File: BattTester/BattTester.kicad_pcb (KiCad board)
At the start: 2 copper layers, 25 parts, among them J1 Battery, J2 SD_Card, J3 PWR, J4 UPDI, Q1 IRLZ44N, U1 LT1286CN8, U2 ATtiny1624-SS, U3 LD1086DT33, U4 LM358AN

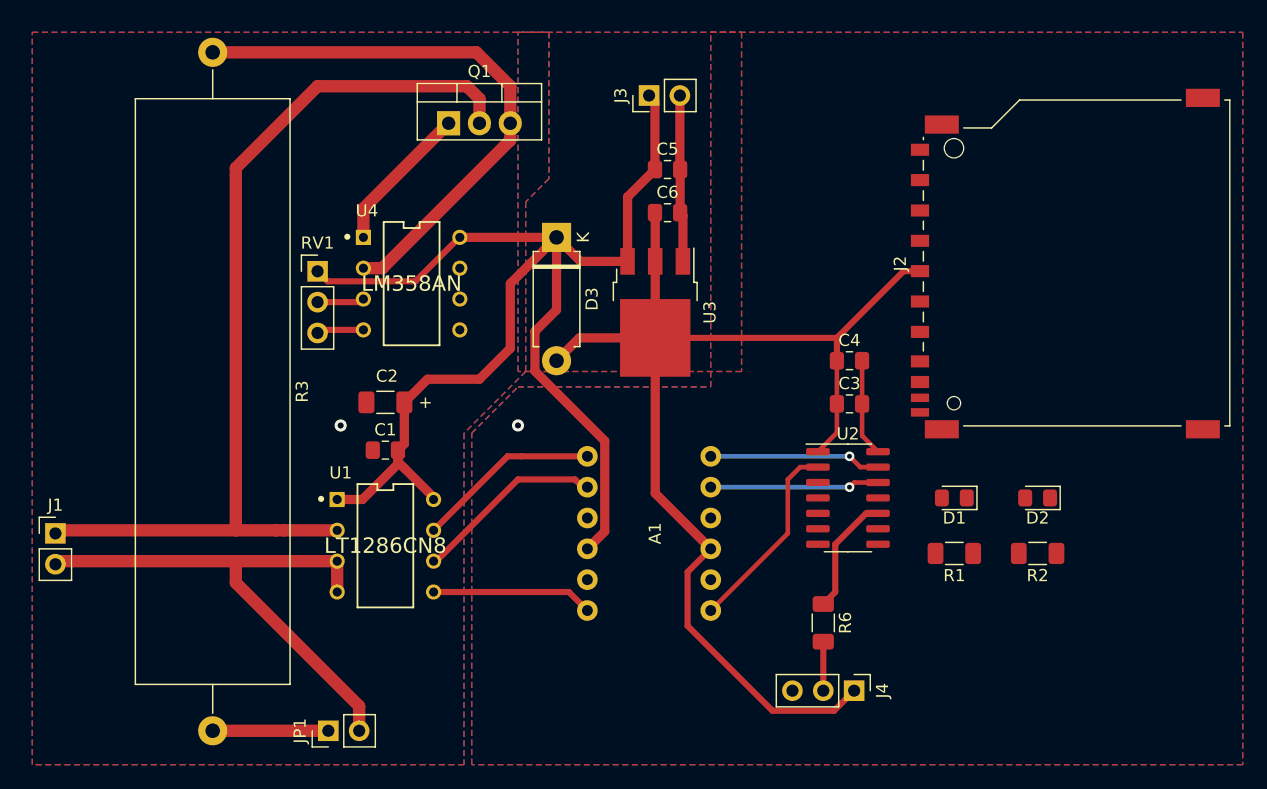
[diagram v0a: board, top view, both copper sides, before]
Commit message: Finish routing
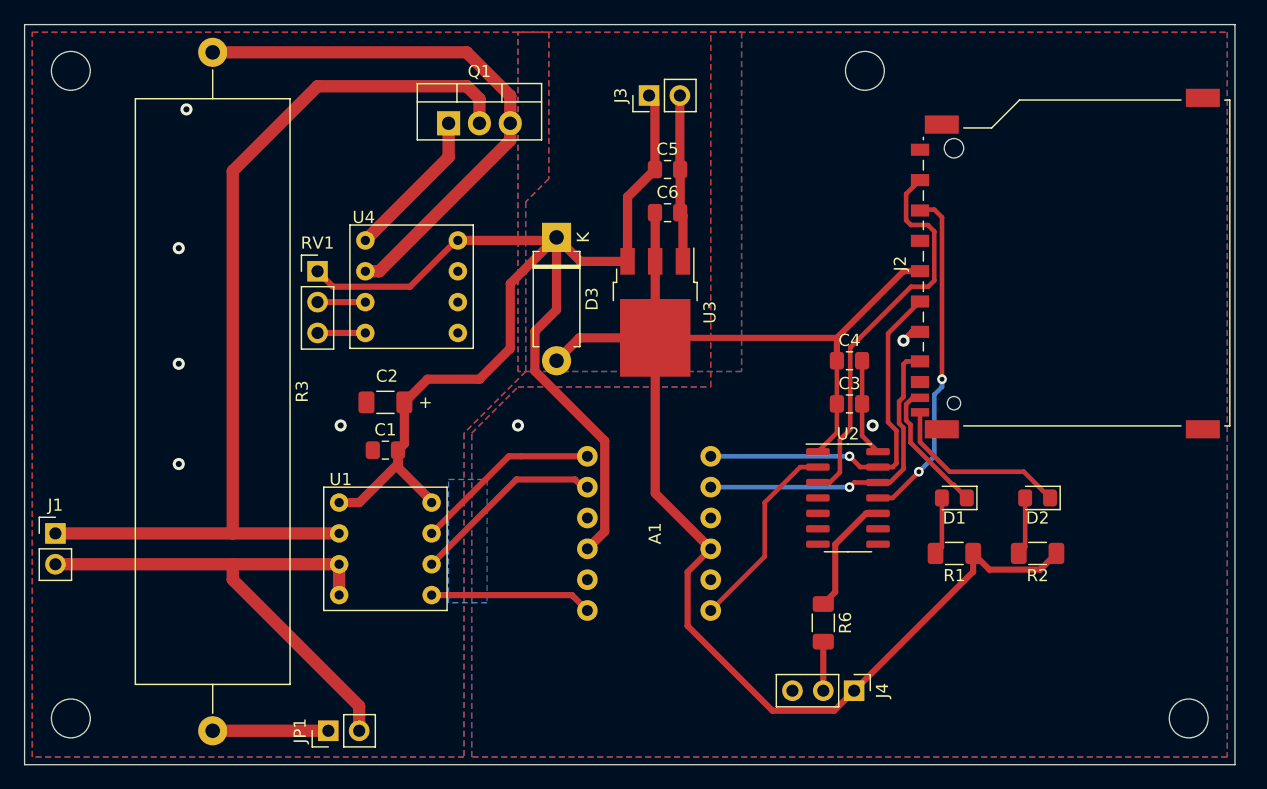
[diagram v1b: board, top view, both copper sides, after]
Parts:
- added REF**: MountingHole_3.2mm_M3, MountingHole:MountingHole_3.2mm_M3, F.Cu at (208.3, 68.6)
- added REF**: MountingHole_3.2mm_M3, MountingHole:MountingHole_3.2mm_M3, F.Cu at (142.9, 68.6)
- added REF**: MountingHole_3.2mm_M3, MountingHole:MountingHole_3.2mm_M3, F.Cu at (142.9, 121.9)
- added REF**: MountingHole_3.2mm_M3, MountingHole:MountingHole_3.2mm_M3, F.Cu at (234.9, 121.9)
- U1, U4: footprint BattTester:Texas_Instruments-P0008A-0-0-MFG -> BattTester:DIP8
- moved U1 4.83 mm to (168.8, 102.9)
- moved U4 4.83 mm to (170.9, 81.3)
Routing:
- net /SPI-CS1: track 0.00 -> 32.5 mm
- net /SPI-MOSI: track 0.00 -> 28.1 mm, vias 0 -> 2
- net +3V3: track 97.0 -> 120.4 mm
- net /SPI-SCK: track 14.1 -> 30.5 mm
- net /WRPrt: track 0.00 -> 15.1 mm
- net /SPI-MISO: track 13.9 -> 26.9 mm
- net /SDDet: track 0.00 -> 11.2 mm
- net Net-(D2-Pad2): track 0.00 -> 4.79 mm
- net Net-(D1-Pad2): track 0.00 -> 4.79 mm
- net GND: track 69.7 -> 71.3 mm, vias 2 -> 8
- net +9V: track 109.5 -> 110.1 mm
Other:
- board outline added: 99.7 x 61 mm

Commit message: minor name fix
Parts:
- U1: value LT1286CN8 -> LTC1286CN8
